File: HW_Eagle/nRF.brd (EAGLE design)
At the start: 37.8 x 34.8 mm, 9 parts, among them X1 B4B-ZR

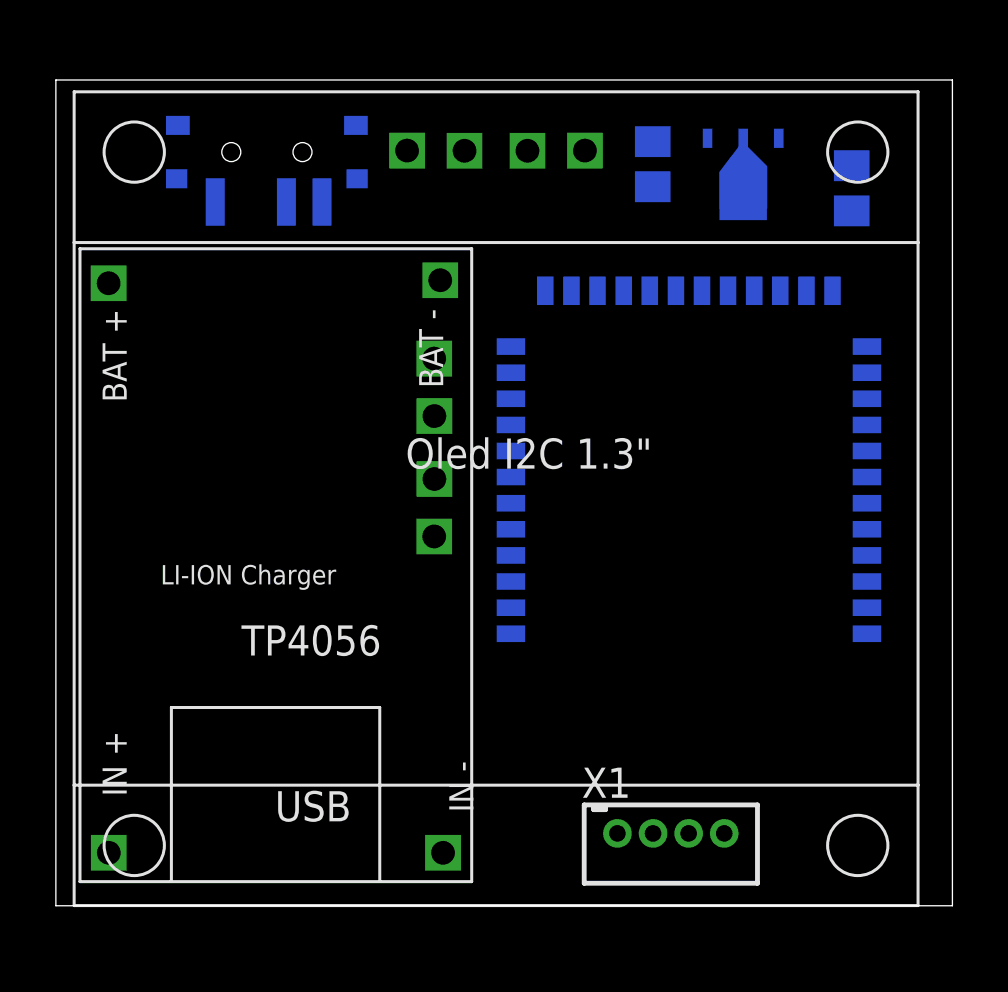
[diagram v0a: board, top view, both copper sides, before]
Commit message: [HW] Update HW v1.2
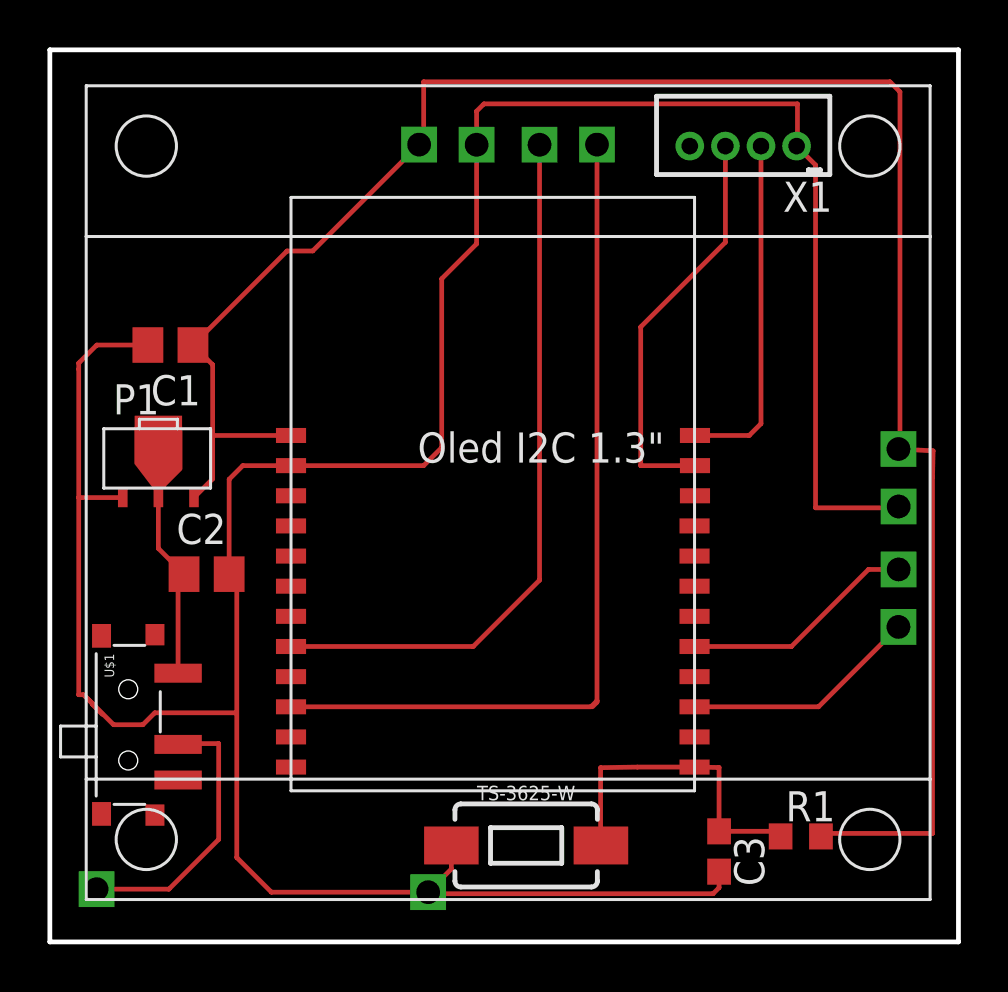
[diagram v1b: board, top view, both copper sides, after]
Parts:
- removed U$2: TP4056, TP4056 charging module:TP4056
- removed U4: (no value), YJ-14015:YJ-14015
- added C3: (no value), rcl:C0603
- added R1: (no value), rcl:R0603
- added TS-3625-W: MOMENTARY-SWITCH-SPST-SMD-6.0X3.5MM, SparkFun-Switches:TACTILE_SWITCH_SMD_6.0X3.5MM
- added U$5: NRF51822, nrf51822:NRF51822_HSHOP
- added U$6: TP4056, TP4056 charging module:TP4056
- moved C2 31.7 mm to (17.5, 52.3), flipped to the top, turned to 0 degrees
- moved X1 29.1 mm to (40.1, 70.4), turned to 180 degrees
- moved P1 27.4 mm to (15.5, 57.1), flipped to the top, turned to 0 degrees
- moved U$1 24.8 mm to (14.2, 46.0), flipped to the top, turned to 270 degrees
- moved C1 21.7 mm to (16.0, 62.0), flipped to the top, turned to 180 degrees
- moved U$4 19.9 mm to (40.4, 51.3)
- moved U$3 0.57 mm to (27.7, 60.2)
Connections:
- new net BUTTON: C3.1, R1.1, TS-3625-W.2, U$5.P$13
- net GND: now also C3.2, TS-3625-W.1, U$5.P$11, U$6.BAT-; no longer U$2.BAT-, U4.GND, U4.GND@2
- net MPU6050_SCL: now also U$5.P$17; no longer U4.P.04
- net MPU6050_SDA: now also U$5.P$15; no longer U4.P.07
- net N$1: now also U$6.BAT+; no longer U$2.BAT+
- net OLED_SCL: now also U$5.P$5; no longer U4.P.24
- net OLED_SDA: now also U$5.P$3; no longer U4.P.22
- net SWDCLK: now also U$5.P$24; no longer U4.SWDCLK
- net SWDIO: now also U$5.P$23; no longer U4.SWDIO
- net VCC: now also R1.2, U$5.P$12; no longer U4.VDD
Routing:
- net GND: track 0.00 -> 126.6 mm
- net VCC: track 0.00 -> 83.8 mm
- net OLED_SDA: track 0.00 -> 36.8 mm
- net OLED_SCL: track 0.00 -> 30.0 mm
- net SWDIO: track 0.00 -> 17.2 mm
- net SWDCLK: track 0.00 -> 14.7 mm
- net BUTTON: track 0.00 -> 13.6 mm
- net N$1: track 0.00 -> 11.8 mm
- net MPU6050_SDA: track 0.00 -> 9.98 mm
- net MPU6050_SCL: track 0.00 -> 9.94 mm
- net V_BAT: track 0.00 -> 7.98 mm
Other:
- board size 37.8 x 34.8 mm -> 38.3 x 37.6 mm
